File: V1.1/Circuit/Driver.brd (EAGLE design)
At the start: 61.6 x 54.6 mm, 32 parts, among them IC1 DRV8300DIPWR, IC2 CD74HC4049PWR, U1 INA240A1PWR, U2 INA240A1PWR, U3 INA240A1PWR

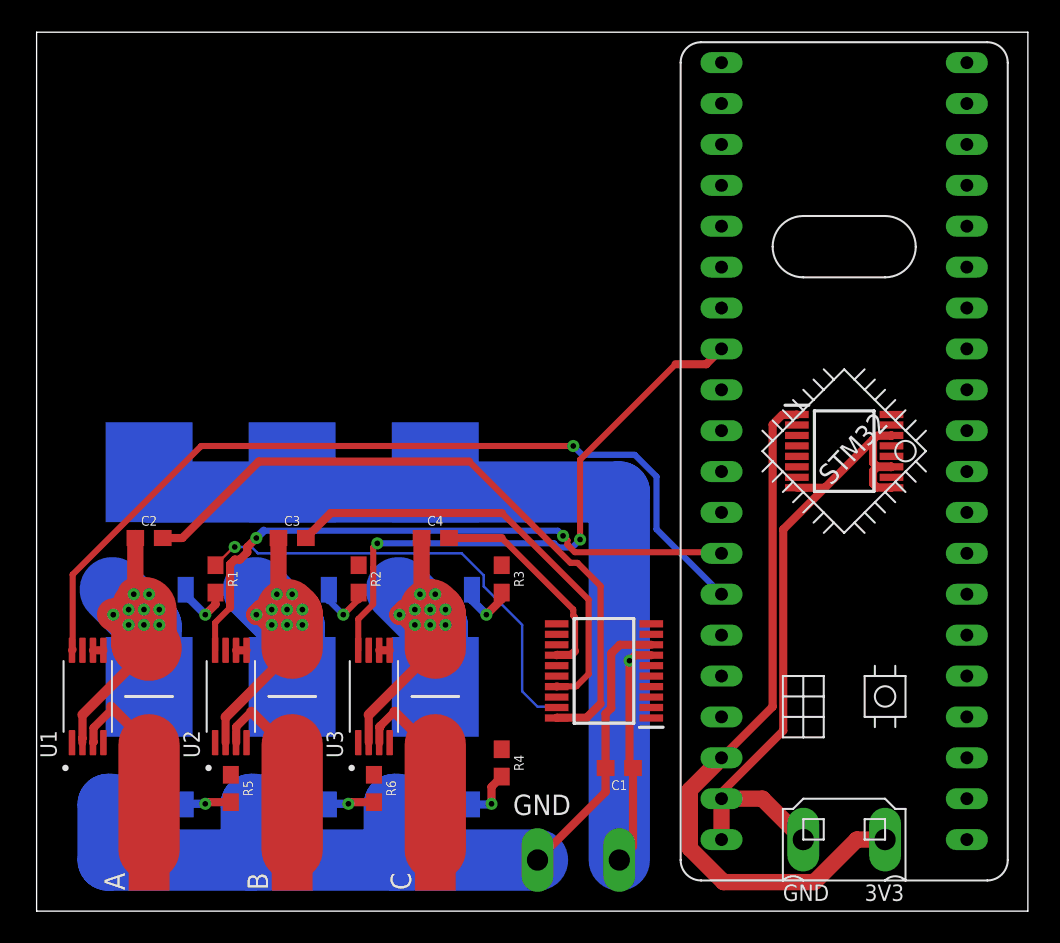
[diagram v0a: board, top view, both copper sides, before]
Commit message: Ready for autoroutering 6
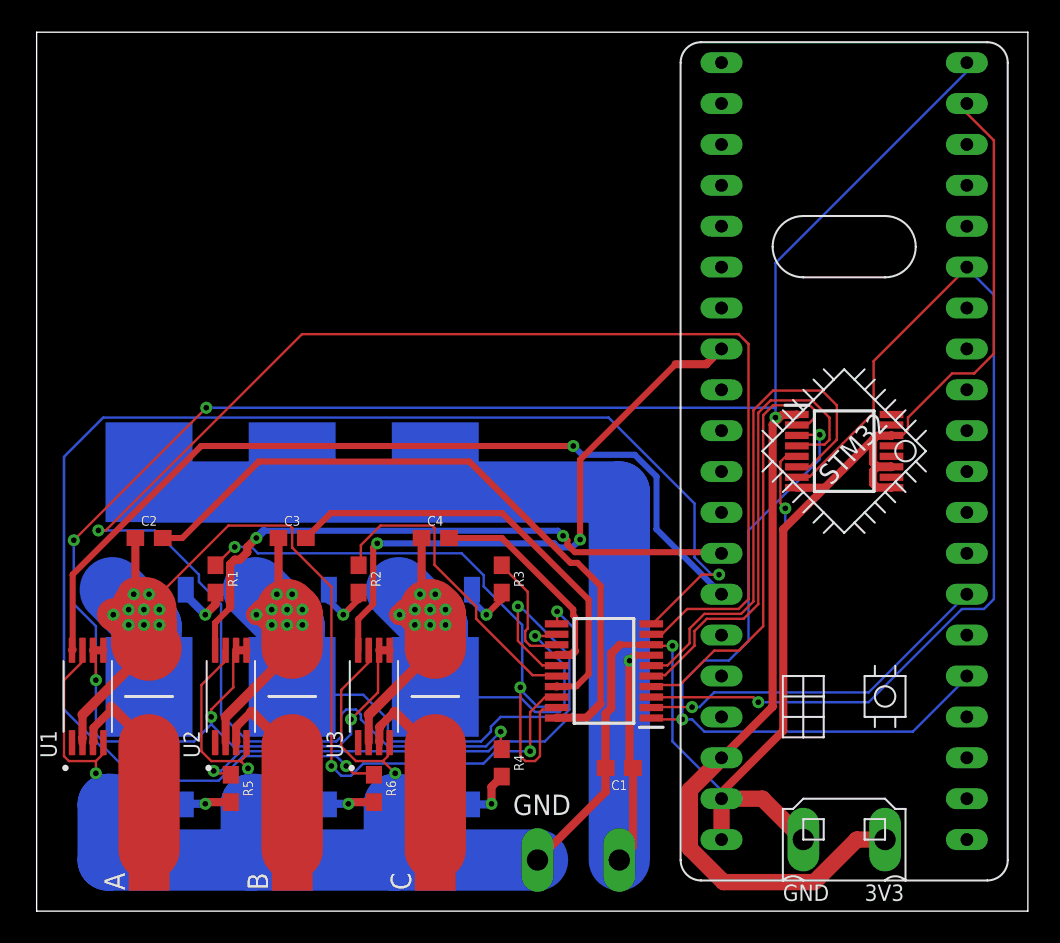
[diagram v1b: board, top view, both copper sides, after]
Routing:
- net 3V3: track 46.3 -> 163.5 mm, vias 0 -> 6
- net GLC: track 0.00 -> 107.4 mm, vias 0 -> 2
- net GLB: track 0.00 -> 91.1 mm, vias 0 -> 2
- net GND: track 99.1 -> 177.5 mm, vias 0 -> 4
- net INHC: track 0.00 -> 63.3 mm, vias 0 -> 1
- net SHA: track 28.6 -> 78.4 mm, vias 9 -> 11
- net INHA: track 0.00 -> 45.0 mm, vias 0 -> 2
- net SHB: track 25.0 -> 65.5 mm, vias 9 -> 10
- net INHB: track 0.00 -> 38.1 mm, vias 0 -> 2
- net GLA: track 0.00 -> 32.6 mm, vias 0 -> 2
- net INLC: track 0.00 -> 31.8 mm
- net INLB: track 0.00 -> 29.7 mm
- net INLA: track 0.00 -> 27.0 mm
- net SHC: track 25.0 -> 47.7 mm, vias 9 -> 10
- net GHB: track 0.00 -> 19.7 mm
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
